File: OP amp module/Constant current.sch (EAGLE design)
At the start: 6 parts, among them IC1 LM358N

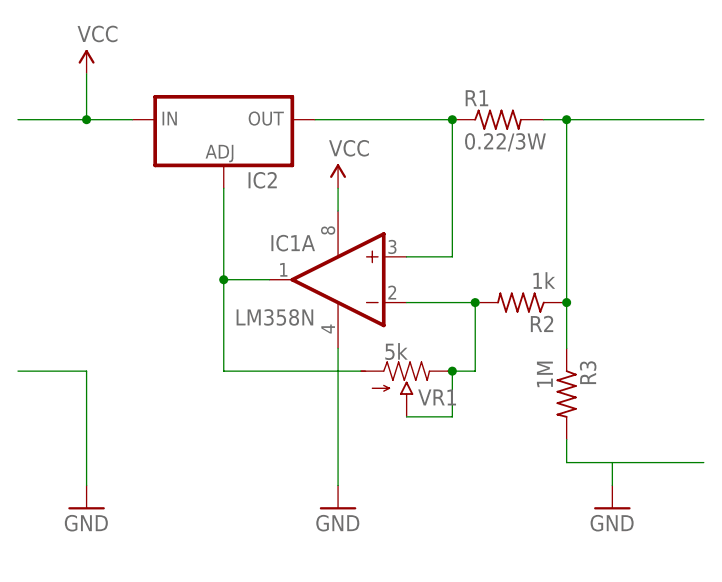
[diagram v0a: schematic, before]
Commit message: Constant current
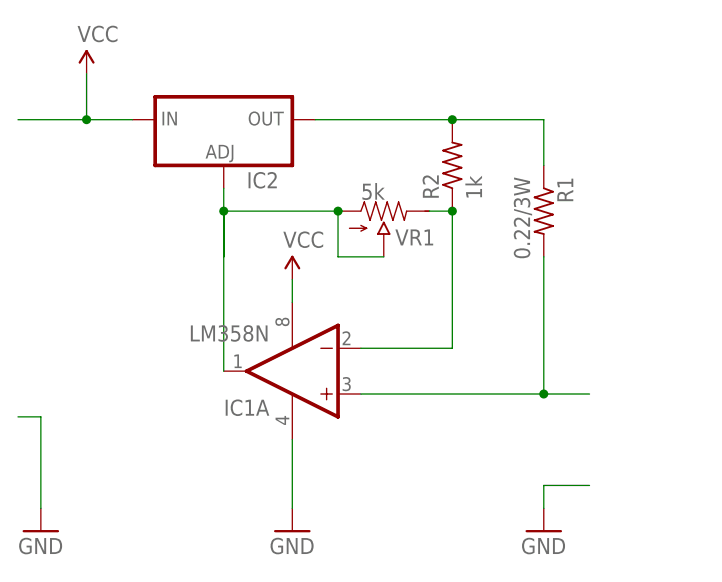
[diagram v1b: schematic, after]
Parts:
- removed R3: 1M, rcl:R-US_0414/15
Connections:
- removed net N$1: IC1A.+IN, IC2.OUT, R1.1
- removed net N$5: IC1A.-IN, R2.2, VR1.E, VR1.S
- new net N$2: IC1A.OUT, IC2.ADJ, VR1.A, VR1.S
- new net N$4: IC2.OUT, R1.1, R2.2
- net GND: no longer R3.2
- net N$3: now also IC1A.-IN, R2.1, VR1.E; no longer IC1A.OUT, IC2.ADJ, VR1.A
- net N$6: now also IC1A.+IN; no longer R2.1, R3.1
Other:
- moved on the sheet: IC1A, R1, R2, VR1
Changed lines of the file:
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@@
 <part name="VR1" library="My Library" deviceset="POT" device="100K_3362U" value="5k"/>
 <part name="R2" library="rcl" deviceset="R-US_" device="0414/15" value="1k"/>
-<part name="R3" library="rcl" deviceset="R-US_" device="0414/15" value="1M"/>
 </parts>
 <sheets>
@@
 </plain>
 <instances>
-<instance part="IC1" gate="A" x="40.64" y="55.88" rot="MR0"/>
+<instance part="IC1" gate="A" x="35.56" y="45.72" rot="R180"/>
 <instance part="IC2" gate="1" x="27.94" y="73.66"/>
-<instance part="R1" gate="G$1" x="58.42" y="73.66"/>
+<instance part="R1" gate="G$1" x="63.5" y="63.5" rot="R270"/>
 <instance part="P+1" gate="1" x="12.7" y="78.74"/>
-<instance part="IC1" gate="P" x="40.64" y="55.88"/>
-<instance part="P+2" gate="1" x="40.64" y="66.04"/>
-<instance part="GND1" gate="1" x="40.64" y="30.48"/>
-<instance part="GND2" gate="1" x="71.12" y="30.48"/>
-<instance part="GND3" gate="1" x="12.7" y="30.48"/>
-<instance part="VR1" gate="G$1" x="48.26" y="45.72" rot="R270"/>
-<instance part="R2" gate="G$1" x="60.96" y="53.34" rot="R180"/>
-<instance part="R3" gate="G$1" x="66.04" y="43.18" rot="R270"/>
+<instance part="IC1" gate="P" x="35.56" y="45.72"/>
+<instance part="P+2" gate="1" x="35.56" y="55.88"/>
+<instance part="GND1" gate="1" x="35.56" y="27.94"/>
+<instance part="GND2" gate="1" x="63.5" y="27.94"/>
+<instance part="GND3" gate="1" x="7.62" y="27.94"/>
+<instance part="VR1" gate="G$1" x="45.72" y="63.5" rot="R270"/>
+<instance part="R2" gate="G$1" x="53.34" y="68.58" rot="R90"/>
 </instances>
 <busses>
 </busses>
 <nets>
-<net name="N$1" class="0">
-<segment>
-<pinref part="IC2" gate="1" pin="OUT"/>
-<pinref part="R1" gate="G$1" pin="1"/>
-<wire x1="38.1" y1="73.66" x2="53.34" y2="73.66" width="0.1524" layer="91"/>
-<wire x1="53.34" y1="73.66" x2="53.34" y2="58.42" width="0.1524" layer="91"/>
-<pinref part="IC1" gate="A" pin="+IN"/>
-<wire x1="53.34" y1="58.42" x2="48.26" y2="58.42" width="0.1524" layer="91"/>
-<junction x="53.34" y="73.66"/>
-</segment>
-</net>
-<net name="N$3" class="0">
-<segment>
-<pinref part="IC2" gate="1" pin="ADJ"/>
-<wire x1="27.94" y1="66.04" x2="27.94" y2="55.88" width="0.1524" layer="91"/>
-<pinref part="IC1" gate="A" pin="OUT"/>
-<wire x1="27.94" y1="55.88" x2="33.02" y2="55.88" width="0.1524" layer="91"/>
-<wire x1="43.18" y1="45.72" x2="27.94" y2="45.72" width="0.1524" layer="91"/>
-<wire x1="27.94" y1="45.72" x2="27.94" y2="55.88" width="0.1524" layer="91"/>
-<junction x="27.94" y="55.88"/>
-<pinref part="VR1" gate="G$1" pin="A"/>
-</segment>
-</net>
 <net name="VCC" class="0">
 <segment>
@@
 <pinref part="P+2" gate="1" pin="VCC"/>
 <pinref part="IC1" gate="P" pin="V+"/>
-<wire x1="40.64" y1="66.04" x2="40.64" y2="63.5" width="0.1524" layer="91"/>
+<wire x1="35.56" y1="55.88" x2="35.56" y2="53.34" width="0.1524" layer="91"/>
 </segment>
 </net>
@@
 <pinref part="IC1" gate="P" pin="V-"/>
 <pinref part="GND1" gate="1" pin="GND"/>
-<wire x1="40.64" y1="48.26" x2="40.64" y2="33.02" width="0.1524" layer="91"/>
+<wire x1="35.56" y1="38.1" x2="35.56" y2="30.48" width="0.1524" layer="91"/>
 </segment>
 <segment>
-<wire x1="81.28" y1="35.56" x2="71.12" y2="35.56" width="0.1524" layer="91"/>
+<wire x1="68.58" y1="33.02" x2="63.5" y2="33.02" width="0.1524" layer="91"/>
 <pinref part="GND2" gate="1" pin="GND"/>
-<wire x1="71.12" y1="35.56" x2="71.12" y2="33.02" width="0.1524" layer="91"/>
-<pinref part="R3" gate="G$1" pin="2"/>
-<wire x1="71.12" y1="35.56" x2="66.04" y2="35.56" width="0.1524" layer="91"/>
-<wire x1="66.04" y1="35.56" x2="66.04" y2="38.1" width="0.1524" layer="91"/>
+<wire x1="63.5" y1="33.02" x2="63.5" y2="30.48" width="0.1524" layer="91"/>
 </segment>
 <segment>
 <pinref part="GND3" gate="1" pin="GND"/>
-<wire x1="12.7" y1="33.02" x2="12.7" y2="45.72" width="0.1524" layer="91"/>
-<wire x1="12.7" y1="45.72" x2="5.08" y2="45.72" width="0.1524" layer="91"/>
+<wire x1="7.62" y1="30.48" x2="7.62" y2="40.64" width="0.1524" layer="91"/>
+<wire x1="7.62" y1="40.64" x2="5.08" y2="40.64" width="0.1524" layer="91"/>
 </segment>
 </net>
 <net name="N$6" class="0">
 <segment>
-<pinref part="R2" gate="G$1" pin="1"/>
 <pinref part="R1" gate="G$1" pin="2"/>
-<wire x1="63.5" y1="73.66" x2="66.04" y2="73.66" width="0.1524" layer="91"/>
-<wire x1="66.04" y1="73.66" x2="81.28" y2="73.66" width="0.1524" layer="91"/>
-<wire x1="66.04" y1="53.34" x2="66.04" y2="73.66" width="0.1524" layer="91"/>
-<junction x="66.04" y="73.66"/>
-<pinref part="R3" gate="G$1" pin="1"/>
-<wire x1="66.04" y1="48.26" x2="66.04" y2="53.34" width="0.1524" layer="91"/>
-<junction x="66.04" y="53.34"/>
+<wire x1="63.5" y1="58.42" x2="63.5" y2="43.18" width="0.1524" layer="91"/>
+<pinref part="IC1" gate="A" pin="+IN"/>
+<wire x1="63.5" y1="43.18" x2="68.58" y2="43.18" width="0.1524" layer="91"/>
+<wire x1="43.18" y1="43.18" x2="63.5" y2="43.18" width="0.1524" layer="91"/>
+<junction x="63.5" y="43.18"/>
 </segment>
 </net>
-<net name="N$5" class="0">
+<net name="N$2" class="0">
 <segment>
-<wire x1="55.88" y1="45.72" x2="53.34" y2="45.72" width="0.1524" layer="91"/>
-<pinref part="IC1" gate="A" pin="-IN"/>
-<pinref part="R2" gate="G$1" pin="2"/>
-<wire x1="48.26" y1="53.34" x2="55.88" y2="53.34" width="0.1524" layer="91"/>
-<wire x1="55.88" y1="45.72" x2="55.88" y2="53.34" width="0.1524" layer="91"/>
-<junction x="55.88" y="53.34"/>
+<pinref part="IC1" gate="A" pin="OUT"/>
+<wire x1="27.94" y1="45.72" x2="27.94" y2="63.5" width="0.1524" layer="91"/>
+<pinref part="VR1" gate="G$1" pin="A"/>
+<wire x1="27.94" y1="63.5" x2="40.64" y2="63.5" width="0.1524" layer="91"/>
+<pinref part="IC2" gate="1" pin="ADJ"/>
+<wire x1="27.94" y1="66.04" x2="27.94" y2="63.5" width="0.1524" layer="91"/>
+<wire x1="27.94" y1="63.5" x2="27.94" y2="58.42" width="0.1524" layer="91"/>
+<wire x1="27.94" y1="58.42" x2="27.94" y2="63.5" width="0.1524" layer="91"/>
 <pinref part="VR1" gate="G$1" pin="S"/>
-<wire x1="48.26" y1="40.64" x2="53.34" y2="40.64" width="0.1524" layer="91"/>
-<wire x1="53.34" y1="40.64" x2="53.34" y2="45.72" width="0.1524" layer="91"/>
-<pinref part="VR1" gate="G$1" pin="E"/>
-<junction x="53.34" y="45.72"/>
+<wire x1="45.72" y1="58.42" x2="40.64" y2="58.42" width="0.1524" layer="91"/>
+<wire x1="40.64" y1="58.42" x2="40.64" y2="63.5" width="0.1524" layer="91"/>
+<junction x="27.94" y="63.5"/>
+<junction x="40.64" y="63.5"/>
 </segment>
 </net>
+<net name="N$3" class="0">
+<segment>
+<pinref part="VR1" gate="G$1" pin="E"/>
+<pinref part="R2" gate="G$1" pin="1"/>
+<wire x1="50.8" y1="63.5" x2="53.34" y2="63.5" width="0.1524" layer="91"/>
+<wire x1="53.34" y1="63.5" x2="53.34" y2="48.26" width="0.1524" layer="91"/>
+<pinref part="IC1" gate="A" pin="-IN"/>
+<wire x1="53.34" y1="48.26" x2="43.18" y2="48.26" width="0.1524" layer="91"/>
+<junction x="53.34" y="63.5"/>
+</segment>
+</net>
+<net name="N$4" class="0">
+<segment>
+<pinref part="IC2" gate="1" pin="OUT"/>
+<pinref part="R2" gate="G$1" pin="2"/>
+<wire x1="38.1" y1="73.66" x2="53.34" y2="73.66" width="0.1524" layer="91"/>
+<wire x1="53.34" y1="73.66" x2="63.5" y2="73.66" width="0.1524" layer="91"/>
+<wire x1="63.5" y1="73.66" x2="63.5" y2="68.58" width="0.1524" layer="91"/>
+<junction x="53.34" y="73.66"/>
+<pinref part="R1" gate="G$1" pin="1"/>
+</segment>
+</net>
